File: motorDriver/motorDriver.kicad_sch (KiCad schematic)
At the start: 22 parts, among them IC1 TB67H450FNG,EL, IC2 TB67H450FNG,EL, IC3 TB67H450FNG,EL, IC4 TB67H450FNG,EL, J1 Conn_01x12, J3 FL, J4 FR, J5 BL, J6 BR, J7 Conn_01x02

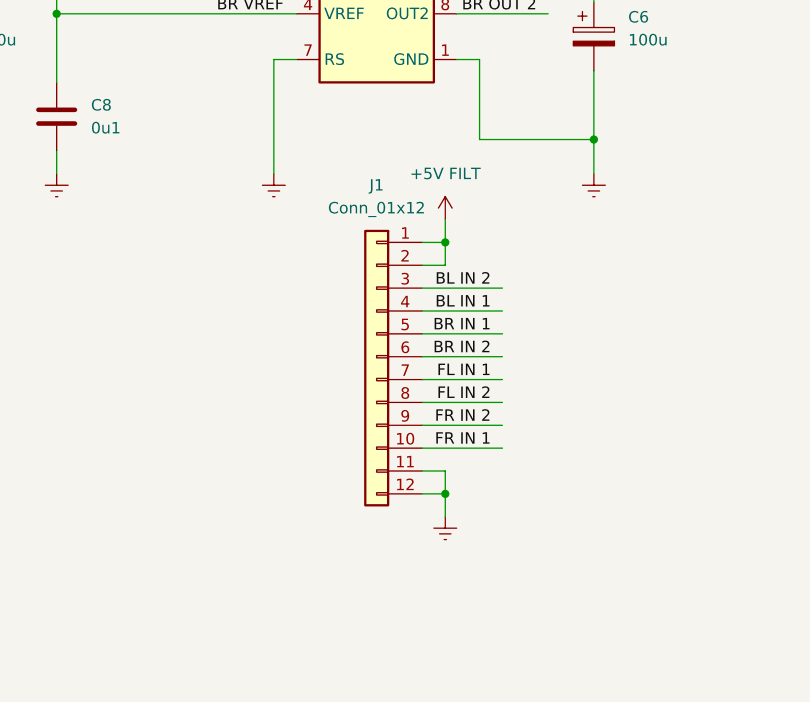
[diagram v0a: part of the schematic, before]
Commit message: 死
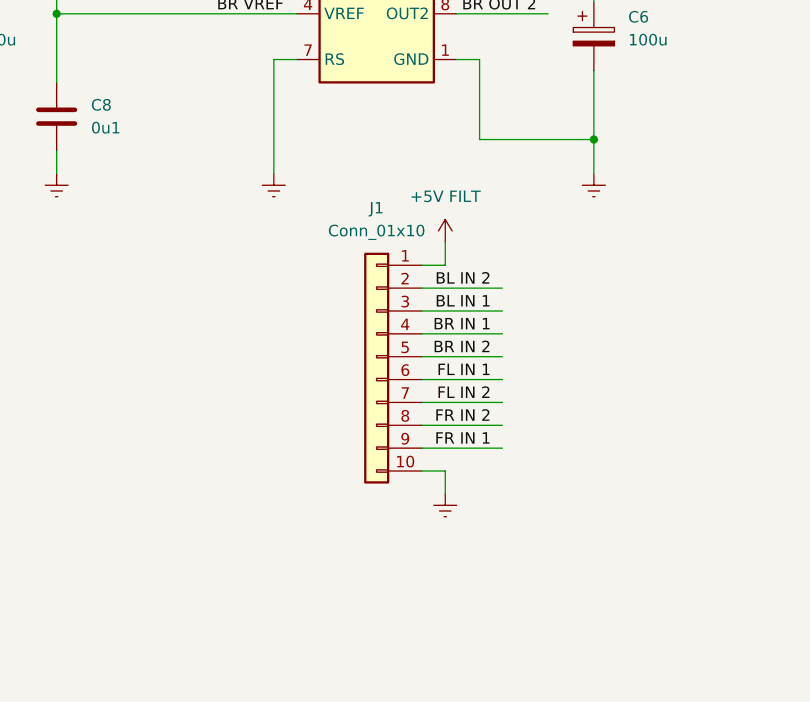
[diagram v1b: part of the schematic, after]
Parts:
- removed J1: Conn_01x12, Library:526101271, symbol Connector_Generic:Conn_01x12
- added J1: Conn_01x10, Library:526101071, symbol Connector_Generic:Conn_01x10
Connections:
- net +5V FILT: now also J1.1 (Pin_1)
- net BL IN 1: now also J1.3 (Pin_3)
- net BL IN 2: now also J1.2 (Pin_2)
- net BR IN 1: now also J1.4 (Pin_4)
- net BR IN 2: now also J1.5 (Pin_5)
- net FL IN 1: now also J1.6 (Pin_6)
- net FL IN 2: now also J1.7 (Pin_7)
- net FR IN 1: now also J1.9 (Pin_9)
- net FR IN 2: now also J1.8 (Pin_8)
- net GNDREF: now also J1.10 (Pin_10)
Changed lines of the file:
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@@
 	)
 	(junction
-		(at 185.42 163.83)
-		(diameter 0)
-		(color 0 0 0 0)
-	)
-	(junction
 		(at 69.85 59.69)
 		(diameter 0)
@@
 	)
 	(junction
-		(at 185.42 135.89)
-		(diameter 0)
-		(color 0 0 0 0)
-	)
-	(junction
 		(at 142.24 110.49)
 		(diameter 0)
@@
 	(wire
 		(pts
-			(xy 182.88 135.89) (xy 185.42 135.89)
-		)
-		(stroke
-			(width 0)
-			(type default)
-		)
-	)
-	(wire
-		(pts
 			(xy 189.23 73.66) (xy 201.93 73.66)
 		)
@@
 	(wire
 		(pts
-			(xy 185.42 135.89) (xy 185.42 133.35)
-		)
-		(stroke
-			(width 0)
-			(type default)
-		)
-	)
-	(wire
-		(pts
 			(xy 69.85 110.49) (xy 69.85 118.11)
 		)
@@
 	(wire
 		(pts
-			(xy 185.42 163.83) (xy 185.42 166.37)
-		)
-		(stroke
-			(width 0)
-			(type default)
-		)
-	)
-	(wire
-		(pts
 			(xy 129.54 46.99) (xy 129.54 50.8)
 		)
@@
 	(wire
 		(pts
-			(xy 182.88 163.83) (xy 185.42 163.83)
-		)
-		(stroke
-			(width 0)
-			(type default)
-		)
-	)
-	(wire
-		(pts
 			(xy 182.88 151.13) (xy 191.77 151.13)
 		)
@@
 	(symbol
 		(lib_id "power:GNDREF")
-		(at 185.42 166.37 0)
+		(at 185.42 163.83 0)
 		(unit 1)
 		(exclude_from_sim no)
@@
 		(fields_autoplaced yes)
 		(property "Reference" "#PWR028"
-			(at 185.42 172.72 0)
+			(at 185.42 170.18 0)
 			(effects
 				(font
@@
 		)
 		(property "Value" "GNDREF"
-			(at 185.42 171.45 0)
+			(at 185.42 168.91 0)
 			(effects
 				(font
@@
 		)
 		(property "Footprint" ""
-			(at 185.42 166.37 0)
+			(at 185.42 163.83 0)
 			(effects
 				(font
@@
 		)
 		(property "Datasheet" ""
-			(at 185.42 166.37 0)
+			(at 185.42 163.83 0)
 			(effects
 				(font
@@
 		)
 		(property "Description" "Power symbol creates a global label with name \"GNDREF\" , reference supply ground"
-			(at 185.42 166.37 0)
+			(at 185.42 163.83 0)
 			(effects
 				(font
@@
 	)
 	(symbol
-		(lib_id "Connector_Generic:Conn_01x12")
+		(lib_id "Connector_Generic:Conn_01x10")
 		(at 177.8 148.59 0)
 		(mirror y)
@@
 		(fields_autoplaced yes)
 		(property "Reference" "J1"
-			(at 177.8 129.54 0)
+			(at 177.8 132.08 0)
 			(effects
 				(font
@@
 			)
 		)
-		(property "Value" "Conn_01x12"
-			(at 177.8 132.08 0)
+		(property "Value" "Conn_01x10"
+			(at 177.8 134.62 0)
 			(effects
 				(font
@@
 			)
 		)
-		(property "Footprint" "Library:526101271"
+		(property "Footprint" "Library:526101071"
 			(at 177.8 148.59 0)
 			(effects
@@
 			)
 		)
-		(property "Description" "Generic connector, single row, 01x12, script generated (kicad-library-utils/schlib/autogen/connector/)"
+		(property "Description" "Generic connector, single row, 01x10, script generated (kicad-library-utils/schlib/autogen/connector/)"
 			(at 177.8 148.59 0)
 			(effects
@@
 		(pin "1"
 		)
-		(pin "6"
+		(pin "5"
 		)
-		(pin "11"
+		(pin "6"
 		)
-		(pin "4"
+		(pin "7"
 		)
 		(pin "9"
 		)
-		(pin "3"
-		)
-		(pin "2"
-		)
-		(pin "7"
-		)
 		(pin "10"
 		)
-		(pin "5"
+		(pin "8"
 		)
-		(pin "12"
+		(pin "2"
 		)
-		(pin "8"
+		(pin "3"
+		)
+		(pin "4"
 		)
 		(instances
@@
 	(symbol
 		(lib_id "power:+5V")
-		(at 185.42 133.35 0)
+		(at 185.42 135.89 0)
 		(unit 1)
 		(exclude_from_sim no)
@@
 		(fields_autoplaced yes)
 		(property "Reference" "#PWR027"
-			(at 185.42 137.16 0)
+			(at 185.42 139.7 0)
 			(effects
 				(font
@@
 		)
 		(property "Value" "+5V FILT"
-			(at 185.42 128.27 0)
+			(at 185.42 130.81 0)
 			(effects
 				(font
@@
 		)
 		(property "Footprint" ""
-			(at 185.42 133.35 0)
+			(at 185.42 135.89 0)
 			(effects
 				(font
@@
 		)
 		(property "Datasheet" ""
-			(at 185.42 133.35 0)
+			(at 185.42 135.89 0)
 			(effects
 				(font
@@
 		)
 		(property "Description" "Power symbol creates a global label with name \"+5V\""
-			(at 185.42 133.35 0)
+			(at 185.42 135.89 0)
 			(effects
 				(font
